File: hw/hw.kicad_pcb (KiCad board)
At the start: 2 copper layers, 58.4 x 78.7 mm, 23 parts, among them J1 Motor 1 Connector, J2 Motor 2 Connector, J3 Distance sensor 3, J4 Distance sensor 1, J5 Distance sensor 2, J6 Distance sensor 6, J7 Distance sensor 4, J8 Distance sensor 5, U1 TB6612FNG_Breakout

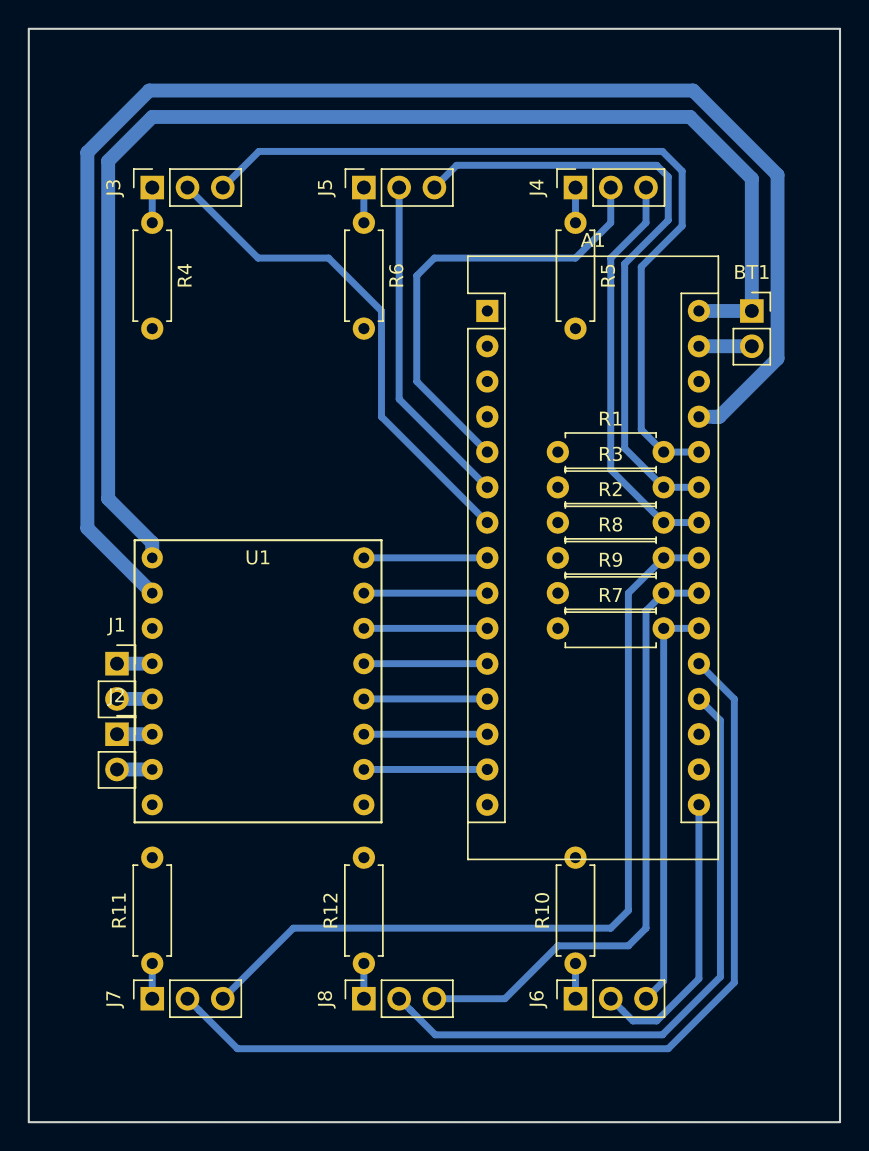
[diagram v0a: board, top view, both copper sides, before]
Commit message: new pcb version
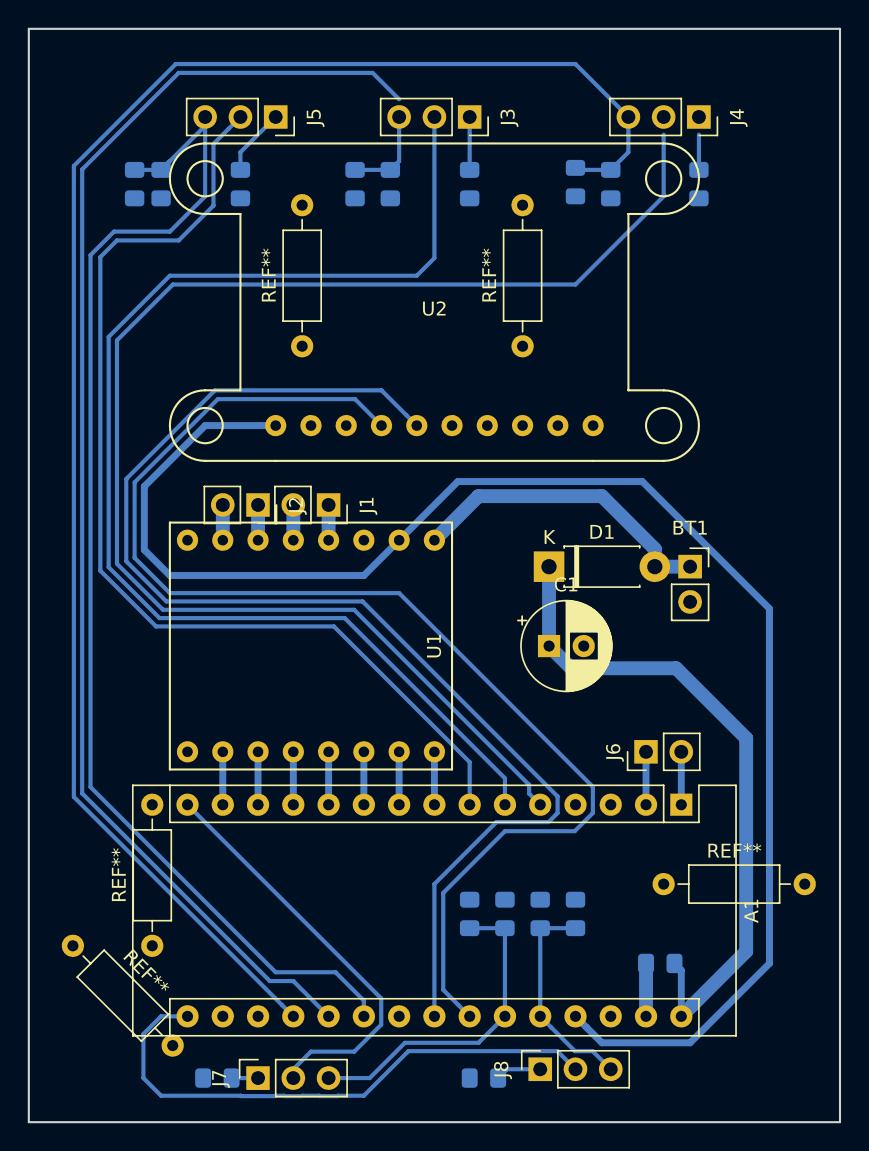
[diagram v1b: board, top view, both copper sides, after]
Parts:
- removed R11, R12: 56, Resistor_THT:R_Axial_DIN0207_L6.3mm_D2.5mm_P7.62mm_Horizontal
- added C1: 100u, Capacitor_THT:CP_Radial_D6.3mm_P2.50mm, F.Cu at (116.2, 92.7)
- added C2: 100n, Capacitor_SMD:C_0805_2012Metric_Pad1.15x1.40mm_HandSolder, B.Cu at (124.2, 115.6)
- added C3: 100n, Capacitor_SMD:C_0805_2012Metric_Pad1.15x1.40mm_HandSolder, B.Cu at (120.7, 59.4)
- added C4: 100n, Capacitor_SMD:C_0805_2012Metric_Pad1.15x1.40mm_HandSolder, B.Cu at (104.8, 59.4)
- added C5: 100n, Capacitor_SMD:C_0805_2012Metric_Pad1.15x1.40mm_HandSolder, B.Cu at (88.3, 59.4)
- added C6: 100n, Capacitor_SMD:C_0805_2012Metric_Pad1.15x1.40mm_HandSolder, B.Cu at (113.0, 112.0)
- added C7: 100n, Capacitor_SMD:C_0805_2012Metric_Pad1.15x1.40mm_HandSolder, B.Cu at (118.1, 112.0)
- added D1: 1N5817, Diode_THT:D_DO-41_SOD81_P7.62mm_Horizontal, F.Cu at (116.2, 87.0)
- added REF**: R_Axial_DIN0207_L6.3mm_D2.5mm_P10.16mm_Horizontal, Resistor_THT:R_Axial_DIN0207_L6.3mm_D2.5mm_P10.16mm_Horizontal, F.Cu at (81.9, 114.3)
- added REF**: R_Axial_DIN0207_L6.3mm_D2.5mm_P10.16mm_Horizontal, Resistor_THT:R_Axial_DIN0207_L6.3mm_D2.5mm_P10.16mm_Horizontal, F.Cu at (114.3, 71.1)
- added REF**: R_Axial_DIN0207_L6.3mm_D2.5mm_P10.16mm_Horizontal, Resistor_THT:R_Axial_DIN0207_L6.3mm_D2.5mm_P10.16mm_Horizontal, F.Cu at (98.4, 71.1)
- added REF**: R_Axial_DIN0207_L6.3mm_D2.5mm_P10.16mm_Horizontal, Resistor_THT:R_Axial_DIN0207_L6.3mm_D2.5mm_P10.16mm_Horizontal, F.Cu at (87.6, 114.3)
- added REF**: R_Axial_DIN0207_L6.3mm_D2.5mm_P10.16mm_Horizontal, Resistor_THT:R_Axial_DIN0207_L6.3mm_D2.5mm_P10.16mm_Horizontal, F.Cu at (124.5, 109.9)
- added U2: L3GD20_breakout, custom:L3GD20_breakout, F.Cu at (108.0, 67.9)
- J3: value Distance sensor 3 -> Distance sensor 2
- J5: value Distance sensor 2 -> Distance sensor 3
- J6: value Distance sensor 6 -> Serial pin header; footprint Connector_PinSocket_2.54mm:PinSocket_1x03_P2.54mm_Vertical -> Connector_PinHeader_2.54mm:PinHeader_1x02_P2.54mm_Vertical
- R1, R2, R3, R7, R9: value 100k -> 1M; footprint Resistor_THT:R_Axial_DIN0207_L6.3mm_D2.5mm_P7.62mm_Horizontal -> Resistor_SMD:R_0805_2012Metric_Pad1.15x1.40mm_HandSolder; moved to B.Cu
- R10, R4, R5, R6: value 56 -> 330; footprint Resistor_THT:R_Axial_DIN0207_L6.3mm_D2.5mm_P7.62mm_Horizontal -> Resistor_SMD:R_0805_2012Metric_Pad1.15x1.40mm_HandSolder; moved to B.Cu
- R8: value 100k -> 330; footprint Resistor_THT:R_Axial_DIN0207_L6.3mm_D2.5mm_P7.62mm_Horizontal -> Resistor_SMD:R_0805_2012Metric_Pad1.15x1.40mm_HandSolder; moved to B.Cu
- moved R8 44.8 mm to (92.3, 123.8), turned to 180 degrees
- moved A1 38.2 mm to (125.7, 104.1), turned to 270 degrees
- moved R3 37.5 mm to (86.4, 59.4), turned to 90 degrees
- moved R2 24.6 mm to (118.1, 59.3), turned to 90 degrees
- moved R1 24.2 mm to (102.2, 59.4), turned to 90 degrees
- moved J3 23.4 mm to (110.5, 54.6), turned to 270 degrees
- moved R9 23.1 mm to (115.6, 112.0), turned to 270 degrees
- moved R4 23.0 mm to (110.5, 59.4)
- moved R7 21.5 mm to (110.5, 112.0), turned to 270 degrees
- moved J2 19.4 mm to (95.2, 82.5), turned to 270 degrees
- moved J1 19.1 mm to (100.3, 82.5), turned to 270 degrees
- moved BT1 18.9 mm to (126.4, 87.0)
- moved J6 18.5 mm to (123.2, 100.3)
- moved U1 17.6 mm to (110.5, 92.7), turned to 270 degrees
- moved J8 13.7 mm to (115.6, 123.2)
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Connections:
- A1 pad 15: Net-(A1-Pad15) -> dist-led-4
- A1 pad 16: dist-led-6 -> dist-led-5
- A1 pad 19: dist-led-5 -> dist-sig-1
- A1 pad 20: dist-led-4 -> dist-sig-2
- A1 pad 21: dist-sig-6 -> dist-sig-3
- A1 pad 22: dist-sig-5 -> Net-(A1-Pad22)
- A1 pad 23: dist-sig-4 -> IMU_SDA
- A1 pad 24: dist-sig-1 -> IMU_SCL
- A1 pad 25: dist-sig-2 -> dist-sig-4
- A1 pad 26: dist-sig-3 -> dist-sig-5
- A1 pad 30: +9V -> V_a
- J3 pad 2: dist-led-3 -> dist-led-2
- J3 pad 3: dist-sig-3 -> dist-sig-2
- J5 pad 2: dist-led-2 -> dist-led-3
- J5 pad 3: dist-sig-2 -> dist-sig-3
- J6 pad 1: Net-(J6-Pad1) -> Net-(A1-Pad2)
- J6 pad 2: dist-led-6 -> Net-(A1-Pad1)
- R1 pad 2: dist-sig-3 -> dist-sig-2
- R10 pad 1: Net-(J6-Pad1) -> Net-(J8-Pad1)
- R3 pad 2: dist-sig-2 -> dist-sig-3
- R7 pad 2: dist-sig-6 -> dist-sig-4
- R8 pad 1: GND -> Net-(J7-Pad1)
- R8 pad 2: dist-sig-4 -> GND
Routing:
- net IMU_SCL: track 0.00 -> 91.0 mm
- net IMU_SDA: track 0.00 -> 90.3 mm
- net dist-sig-1: track 29.3 -> 119.3 mm
- net +9V: track 92.7 -> 22.6 mm
- net dist-led-1: track 32.9 -> 102.3 mm
- net dist-led-2: track 24.2 -> 89.3 mm
- net dist-sig-2: track 45.2 -> 103.1 mm
- net V_a: track 0.00 -> 48.6 mm
- net dist-led-3: track 36.0 -> 74.8 mm
- net dist-sig-4: track 60.8 -> 23.4 mm
- net dist-led-4: track 66.9 -> 29.9 mm
- net dist-sig-3: track 59.4 -> 89.2 mm
- net dist-sig-6: track 29.7 -> 0.00 mm
- net dist-sig-5: track 44.5 -> 15.5 mm
- net dist-led-6: track 20.8 -> 0.00 mm
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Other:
- net class Default: clearance 0.5 -> 0.3
- rule trace_clearance: 0.5 -> 0.3
